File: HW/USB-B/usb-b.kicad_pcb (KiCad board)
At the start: 2 copper layers, 22 x 17 mm, 2 parts

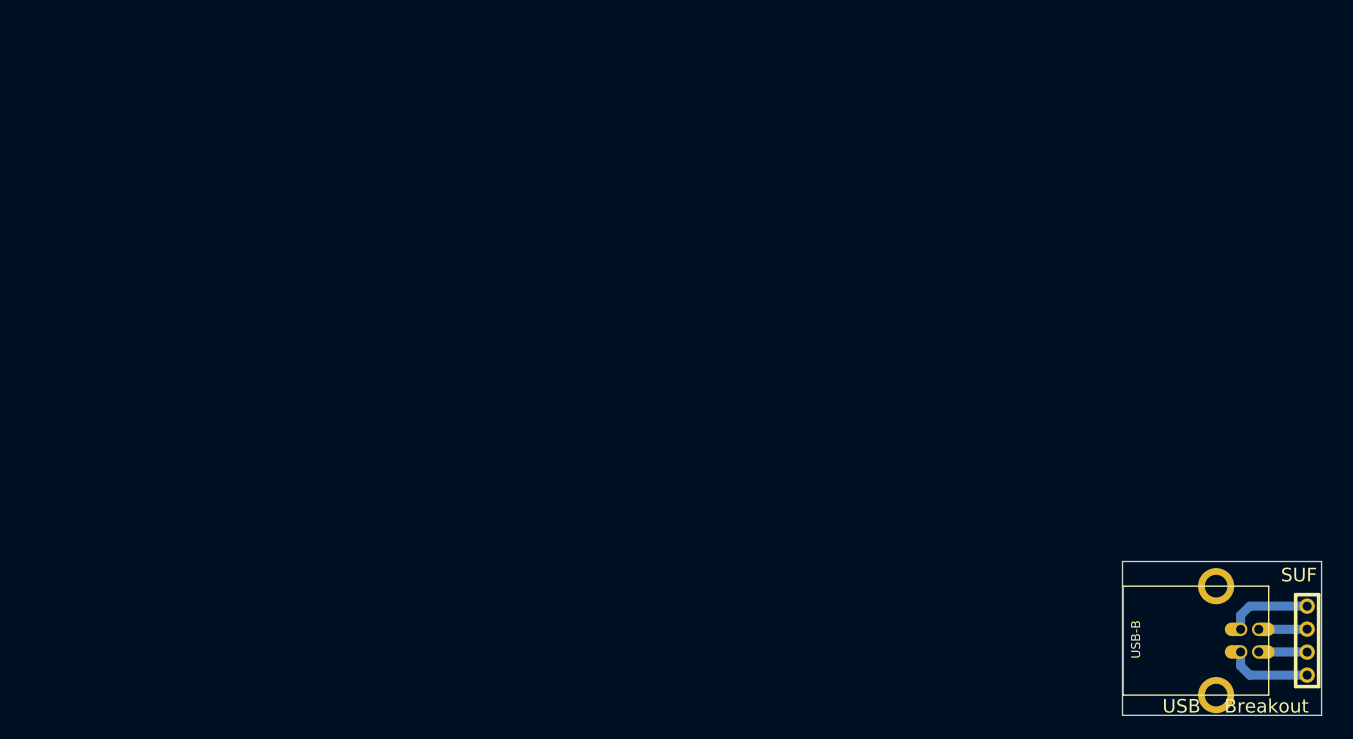
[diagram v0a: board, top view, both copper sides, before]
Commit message: Minor cosmetic corrections
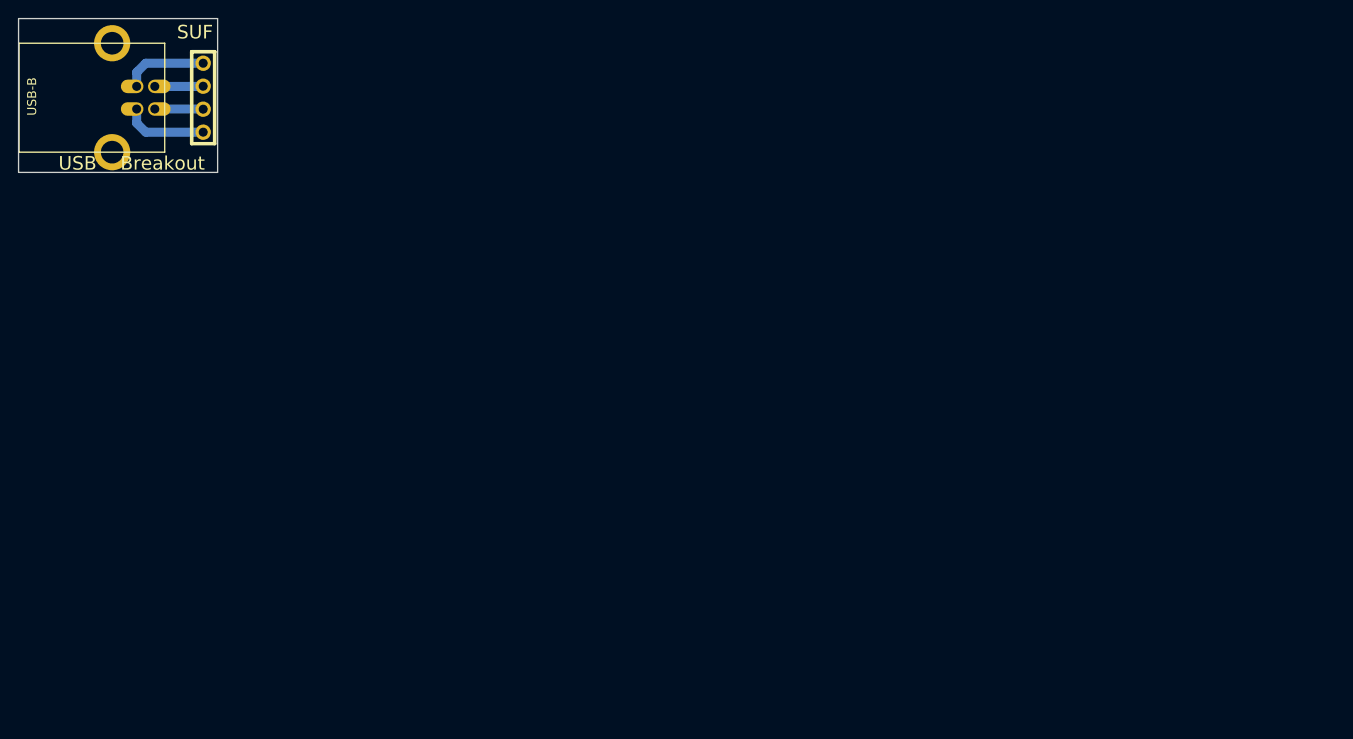
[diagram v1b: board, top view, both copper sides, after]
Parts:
- moved HDR-4 136.0 mm to (70.4, 58.7)
- moved USB-B 136.0 mm to (64.1, 58.7)
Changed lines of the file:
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@@
     (links 0)
     (no_connects 0)
-    (area 0 0 0 0)
+    (area 171.725999 109.949999 196.1134 127.2)
     (thickness 1.6)
     (drawings 21)
@@
     (nets 1)
   )
-  (page A3)
+  (page A4)
   (layers
     (15 F.Cu signal)
@@
   )
   (setup
-    (last_trace_width 1)
+    (last_trace_width 0.254)
     (user_trace_width 0.5)
     (user_trace_width 1)
@@
     (pad_to_mask_clearance 0)
     (aux_axis_origin 0 0)
-    (visible_elements FFFFFFBF)
+    (visible_elements 7FFFFFFF)
     (pcbplotparams
       (layerselection 3178497)
@@
   )
   (module USB-B (layer F.Cu)
-    (at 186.055 118.745 270)
+    (at 64.055 58.745 270)
     (fp_text reference USB-B (at -0.127 12.573 270) (layer F.SilkS)
       (effects (font (size 1 1) (thickness 0.15)))
@@
   )
   (module HDR-4 (layer F.Cu)
-    (at 192.405 118.745 90)
+    (at 70.405 58.745 90)
     (path HDR-5)
     (fp_text reference HDR-4 (at 0 -2.54 90) (layer F.SilkS) hide
@@
     )
   )
-  (gr_text SUF (at 191.5 111.5) (layer F.SilkS)
+  (gr_text SUF (at 69.5 51.5) (layer F.SilkS)
     (effects (font (size 1.5 1.5) (thickness 0.3)))
   )
-  (gr_text "USB    Breakout" (at 184.5 126) (layer F.SilkS)
+  (gr_text "USB    Breakout" (at 62.5 66) (layer F.SilkS)
     (effects (font (size 1.5 1.5) (thickness 0.3)))
   )
-  (gr_line (start 172 127) (end 172 110) (angle 90) (layer Edge.Cuts) (width 0.1))
-  (gr_line (start 194 127) (end 172 127) (angle 90) (layer Edge.Cuts) (width 0.1))
-  (gr_line (start 194 110) (end 194 127) (angle 90) (layer Edge.Cuts) (width 0.1))
-  (gr_line (start 172 110) (end 194 110) (angle 90) (layer Edge.Cuts) (width 0.1))
-  (gr_line (start 191.262 115.062) (end 180.594 115.062) (angle 90) (layer B.SilkS) (width 0.2))
-  (gr_line (start 191.262 117.602) (end 180.594 117.602) (angle 90) (layer B.SilkS) (width 0.2))
-  (gr_line (start 191.262 119.888) (end 180.594 119.888) (angle 90) (layer B.SilkS) (width 0.2))
-  (gr_line (start 191.262 122.428) (end 180.594 122.428) (angle 90) (layer B.SilkS) (width 0.2))
-  (gr_line (start 180.594 121.158) (end 174.752 121.158) (angle 90) (layer B.SilkS) (width 0.2))
-  (gr_line (start 180.594 118.618) (end 174.752 118.618) (angle 90) (layer B.SilkS) (width 0.2))
-  (gr_line (start 180.594 116.078) (end 174.752 116.078) (angle 90) (layer B.SilkS) (width 0.2))
-  (gr_line (start 174.752 123.952) (end 174.752 113.538) (angle 90) (layer B.SilkS) (width 0.2))
-  (gr_line (start 180.594 123.952) (end 174.752 123.952) (angle 90) (layer B.SilkS) (width 0.2))
-  (gr_line (start 180.594 113.538) (end 180.594 123.952) (angle 90) (layer B.SilkS) (width 0.2))
-  (gr_line (start 174.752 113.538) (end 180.594 113.538) (angle 90) (layer B.SilkS) (width 0.2))
-  (gr_text GND (at 177.8 122.682) (layer B.SilkS)
+  (gr_line (start 50 67) (end 50 50) (angle 90) (layer Edge.Cuts) (width 0.1))
+  (gr_line (start 72 67) (end 50 67) (angle 90) (layer Edge.Cuts) (width 0.1))
+  (gr_line (start 72 50) (end 72 67) (angle 90) (layer Edge.Cuts) (width 0.1))
+  (gr_line (start 50 50) (end 72 50) (angle 90) (layer Edge.Cuts) (width 0.1))
+  (gr_line (start 69.262 55.062) (end 58.594 55.062) (angle 90) (layer B.SilkS) (width 0.2))
+  (gr_line (start 69.262 57.602) (end 58.594 57.602) (angle 90) (layer B.SilkS) (width 0.2))
+  (gr_line (start 69.262 59.888) (end 58.594 59.888) (angle 90) (layer B.SilkS) (width 0.2))
+  (gr_line (start 69.262 62.428) (end 58.594 62.428) (angle 90) (layer B.SilkS) (width 0.2))
+  (gr_line (start 58.594 61.158) (end 52.752 61.158) (angle 90) (layer B.SilkS) (width 0.2))
+  (gr_line (start 58.594 58.618) (end 52.752 58.618) (angle 90) (layer B.SilkS) (width 0.2))
+  (gr_line (start 58.594 56.078) (end 52.752 56.078) (angle 90) (layer B.SilkS) (width 0.2))
+  (gr_line (start 52.752 63.952) (end 52.752 53.538) (angle 90) (layer B.SilkS) (width 0.2))
+  (gr_line (start 58.594 63.952) (end 52.752 63.952) (angle 90) (layer B.SilkS) (width 0.2))
+  (gr_line (start 58.594 53.538) (end 58.594 63.952) (angle 90) (layer B.SilkS) (width 0.2))
+  (gr_line (start 52.752 53.538) (end 58.594 53.538) (angle 90) (layer B.SilkS) (width 0.2))
+  (gr_text GND (at 55.8 62.682) (layer B.SilkS)
     (effects (font (size 1.5 1.5) (thickness 0.3)) (justify mirror))
   )
-  (gr_text VCC (at 177.8 120.142) (layer B.SilkS)
+  (gr_text VCC (at 55.8 60.142) (layer B.SilkS)
     (effects (font (size 1.5 1.5) (thickness 0.3)) (justify mirror))
   )
-  (gr_text D- (at 178.562 117.602) (layer B.SilkS)
+  (gr_text D- (at 56.562 57.602) (layer B.SilkS)
     (effects (font (size 1.5 1.5) (thickness 0.3)) (justify mirror))
   )
-  (gr_text D+ (at 178.562 115.062) (layer B.SilkS)
+  (gr_text D+ (at 56.562 55.062) (layer B.SilkS)
     (effects (font (size 1.5 1.5) (thickness 0.3)) (justify mirror))
   )
-  (segment (start 187.055 117.495) (end 192.385 117.495) (width 1) (layer B.Cu) (net 0))
-  (segment (start 192.385 117.495) (end 192.405 117.475) (width 1) (layer B.Cu) (net 0))
-  (segment (start 185.055 117.495) (end 185.055 115.935) (width 1) (layer B.Cu) (net 0))
-  (segment (start 186.055 114.935) (end 192.405 114.935) (width 1) (layer B.Cu) (net 0))
-  (segment (start 185.055 115.935) (end 186.055 114.935) (width 1) (layer B.Cu) (net 0))
-  (segment (start 185.055 119.995) (end 185.055 121.555) (width 1) (layer B.Cu) (net 0))
-  (segment (start 186.055 122.555) (end 192.405 122.555) (width 1) (layer B.Cu) (net 0))
-  (segment (start 185.055 121.555) (end 186.055 122.555) (width 1) (layer B.Cu) (net 0))
-  (segment (start 187.055 119.995) (end 192.385 119.995) (width 1) (layer B.Cu) (net 0))
-  (segment (start 192.385 119.995) (end 192.405 120.015) (width 1) (layer B.Cu) (net 0))
+  (segment (start 65.055 57.495) (end 70.385 57.495) (width 1) (layer B.Cu) (net 0))
+  (segment (start 70.385 57.495) (end 70.405 57.475) (width 1) (layer B.Cu) (net 0))
+  (segment (start 63.055 57.495) (end 63.055 55.935) (width 1) (layer B.Cu) (net 0))
+  (segment (start 64.055 54.935) (end 70.405 54.935) (width 1) (layer B.Cu) (net 0))
+  (segment (start 63.055 55.935) (end 64.055 54.935) (width 1) (layer B.Cu) (net 0))
+  (segment (start 63.055 59.995) (end 63.055 61.555) (width 1) (layer B.Cu) (net 0))
+  (segment (start 64.055 62.555) (end 70.405 62.555) (width 1) (layer B.Cu) (net 0))
+  (segment (start 63.055 61.555) (end 64.055 62.555) (width 1) (layer B.Cu) (net 0))
+  (segment (start 65.055 59.995) (end 70.385 59.995) (width 1) (layer B.Cu) (net 0))
+  (segment (start 70.385 59.995) (end 70.405 60.015) (width 1) (layer B.Cu) (net 0))
 )
